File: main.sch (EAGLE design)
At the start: 30 parts, among them IC1 4050D, U1 MCP2551P-SOCKET, U2 STN1110SOCKET-28, Y1 16Mhz

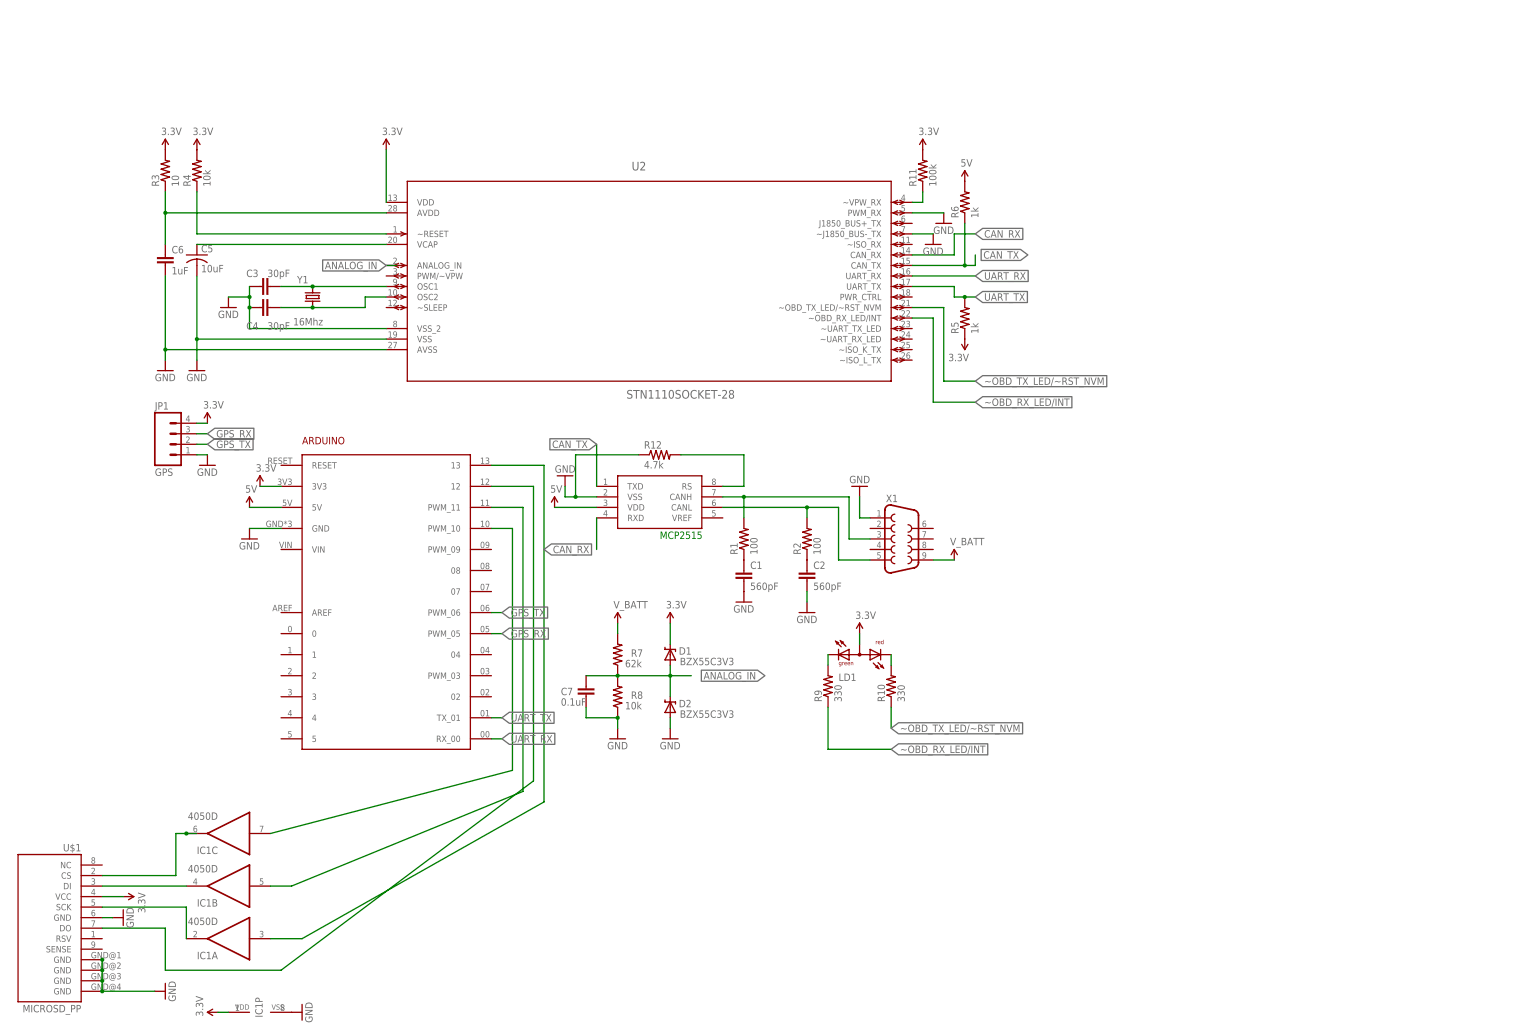
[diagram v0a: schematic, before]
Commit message: Better layout...
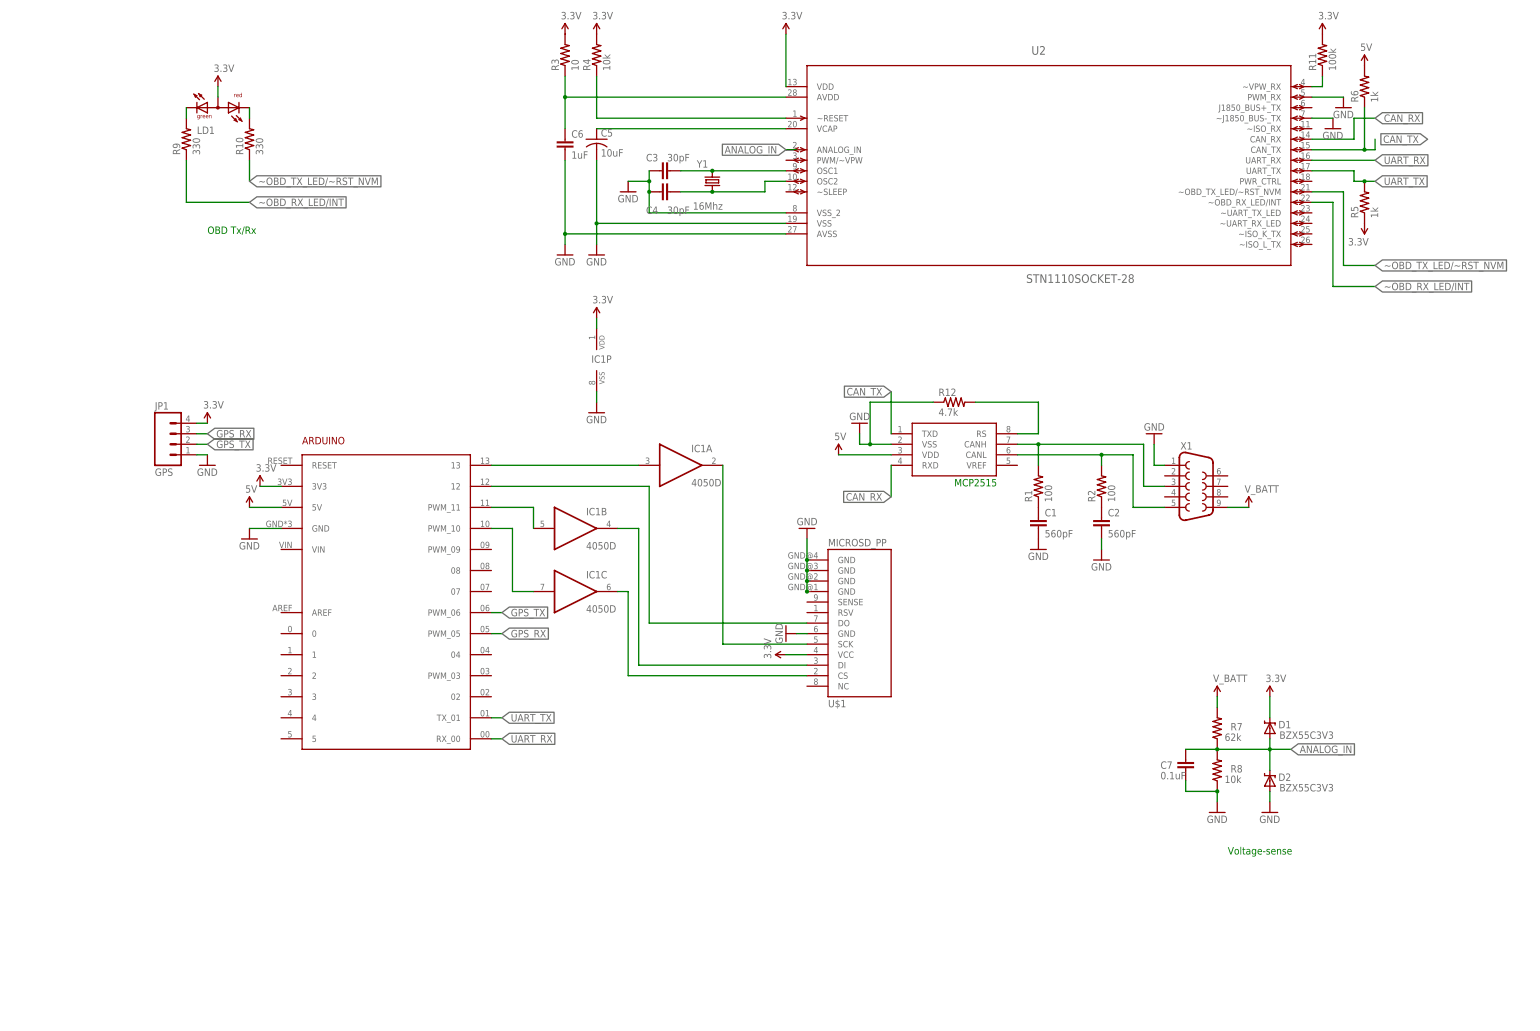
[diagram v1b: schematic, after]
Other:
- note added: "OBD Tx/Rx"
- note added: "Voltage-sense"
- moved on the sheet: C1, C2, C3, C4, C5, C6, C7, D1, D2, IC1A, IC1B, IC1C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
